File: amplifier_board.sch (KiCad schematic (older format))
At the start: 72 parts, among them J1 external input, J10 external saw, J11 jumper storage, J2 AUDIO, J3 VCC, J4 +5V, J5 GND, J6 -5V, J7 audio tune, J8 speaker, J9 speaker, Q1 SQJ860EP, Q2 Q_NMOS_GSD, Q3 SQJ860EP, U1 AD8038, U2 AD8613, U3 LTC4444-5, U4 AD8468, U5 LM555, U6 AD8038, U7 AD8613

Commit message: up
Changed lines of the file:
@@
 L Device:C C17
 U 1 1 5CAB9B8F
-P 2500 5950
-F 0 "C17" V 2375 5875 50  0000 C CNN
-F 1 "100nF" V 2375 6050 50  0000 C CNN
-F 2 "Capacitors_SMD:C_1206_HandSoldering" H 2538 5800 50  0001 C CNN
-F 3 "~" H 2500 5950 50  0001 C CNN
-	1    2500 5950
+P 3175 5950
+F 0 "C17" V 3050 5875 50  0000 C CNN
+F 1 "100nF" V 3050 6050 50  0000 C CNN
+F 2 "Capacitors_SMD:C_1206_HandSoldering" H 3213 5800 50  0001 C CNN
+F 3 "~" H 3175 5950 50  0001 C CNN
+	1    3175 5950
 	-1   0    0    1
 $EndComp
@@
 L Device:C C18
 U 1 1 5CABA0D0
-P 2750 5950
-F 0 "C18" V 2625 5875 50  0000 C CNN
-F 1 "100nF" V 2625 6050 50  0000 C CNN
-F 2 "Capacitors_SMD:C_1206_HandSoldering" H 2788 5800 50  0001 C CNN
-F 3 "~" H 2750 5950 50  0001 C CNN
-	1    2750 5950
+P 3425 5950
+F 0 "C18" V 3300 5875 50  0000 C CNN
+F 1 "100nF" V 3300 6050 50  0000 C CNN
+F 2 "Capacitors_SMD:C_1206_HandSoldering" H 3463 5800 50  0001 C CNN
+F 3 "~" H 3425 5950 50  0001 C CNN
+	1    3425 5950
 	-1   0    0    1
 $EndComp
@@
 L Device:C C19
 U 1 1 5CABA154
-P 3000 5950
-F 0 "C19" V 2875 5875 50  0000 C CNN
-F 1 "100nF" V 2875 6050 50  0000 C CNN
-F 2 "Capacitors_SMD:C_1206_HandSoldering" H 3038 5800 50  0001 C CNN
-F 3 "~" H 3000 5950 50  0001 C CNN
-	1    3000 5950
+P 3675 5950
+F 0 "C19" V 3550 5875 50  0000 C CNN
+F 1 "100nF" V 3550 6050 50  0000 C CNN
+F 2 "Capacitors_SMD:C_1206_HandSoldering" H 3713 5800 50  0001 C CNN
+F 3 "~" H 3675 5950 50  0001 C CNN
+	1    3675 5950
 	-1   0    0    1
 $EndComp
@@
 L Device:C C16
 U 1 1 5CABD33C
-P 2250 5950
-F 0 "C16" V 2125 5875 50  0000 C CNN
-F 1 "100nF" V 2125 6050 50  0000 C CNN
-F 2 "Capacitors_SMD:C_1206_HandSoldering" H 2288 5800 50  0001 C CNN
-F 3 "~" H 2250 5950 50  0001 C CNN
-	1    2250 5950
+P 2925 5950
+F 0 "C16" V 2800 5875 50  0000 C CNN
+F 1 "100nF" V 2800 6050 50  0000 C CNN
+F 2 "Capacitors_SMD:C_1206_HandSoldering" H 2963 5800 50  0001 C CNN
+F 3 "~" H 2925 5950 50  0001 C CNN
+	1    2925 5950
 	-1   0    0    1
 $EndComp
@@
 $EndComp
 Wire Wire Line
-	3000 5800 2750 5800
+	3675 5800 3425 5800
 Connection ~ 1250 5800
 Wire Wire Line
@@
 Wire Wire Line
 	1750 5800 1500 5800
-Connection ~ 2500 5800
-Wire Wire Line
-	2500 5800 2250 5800
-Connection ~ 2750 5800
-Wire Wire Line
-	2750 5800 2500 5800
+Connection ~ 3175 5800
+Wire Wire Line
+	3175 5800 2925 5800
+Connection ~ 3425 5800
+Wire Wire Line
+	3425 5800 3175 5800
 Wire Wire Line
 	1000 5750 1000 5800
@@
 	1500 6100 1750 6100
 Wire Wire Line
-	2250 6100 2500 6100
-Connection ~ 2500 6100
-Wire Wire Line
-	2500 6100 2750 6100
-Connection ~ 2750 6100
-Wire Wire Line
-	2750 6100 3000 6100
+	2925 6100 3175 6100
+Connection ~ 3175 6100
+Wire Wire Line
+	3175 6100 3425 6100
+Connection ~ 3425 6100
+Wire Wire Line
+	3425 6100 3675 6100
 $Comp
 L Device:C C21
@@
 L Device:C C22
 U 1 1 5CAD2A32
-P 1500 6700
-F 0 "C22" V 1375 6625 50  0000 C CNN
-F 1 "100nF" V 1375 6800 50  0000 C CNN
-F 2 "Capacitors_SMD:C_1206_HandSoldering" H 1538 6550 50  0001 C CNN
-F 3 "~" H 1500 6700 50  0001 C CNN
-	1    1500 6700
+P 2000 5950
+F 0 "C22" V 1875 5875 50  0000 C CNN
+F 1 "100nF" V 1875 6050 50  0000 C CNN
+F 2 "Capacitors_SMD:C_1206_HandSoldering" H 2038 5800 50  0001 C CNN
+F 3 "~" H 2000 5950 50  0001 C CNN
+	1    2000 5950
 	-1   0    0    1
 $EndComp
@@
 L Device:C C23
 U 1 1 5CAD2A39
-P 1750 6700
-F 0 "C23" V 1625 6625 50  0000 C CNN
-F 1 "100nF" V 1625 6800 50  0000 C CNN
-F 2 "Capacitors_SMD:C_1206_HandSoldering" H 1788 6550 50  0001 C CNN
-F 3 "~" H 1750 6700 50  0001 C CNN
-	1    1750 6700
+P 2250 5950
+F 0 "C23" V 2125 5875 50  0000 C CNN
+F 1 "100nF" V 2125 6050 50  0000 C CNN
+F 2 "Capacitors_SMD:C_1206_HandSoldering" H 2288 5800 50  0001 C CNN
+F 3 "~" H 2250 5950 50  0001 C CNN
+	1    2250 5950
 	-1   0    0    1
 $EndComp
@@
 $EndComp
 Wire Wire Line
-	1750 6550 1500 6550
-Connection ~ 1250 6550
+	2250 5800 2000 5800
 Wire Wire Line
 	1250 6550 1000 6550
-Connection ~ 1500 6550
-Wire Wire Line
-	1500 6550 1250 6550
+Connection ~ 2000 5800
+Wire Wire Line
+	2000 5800 1750 5800
 Wire Wire Line
 	1000 6850 1250 6850
-Connection ~ 1250 6850
-Wire Wire Line
-	1250 6850 1500 6850
-Connection ~ 1500 6850
-Wire Wire Line
-	1500 6850 1750 6850
+Wire Wire Line
+	1750 6100 2000 6100
+Connection ~ 2000 6100
+Wire Wire Line
+	2000 6100 2250 6100
 $Comp
 L power:GND #PWR0135
@@
 L power:+5V #PWR0101
 U 1 1 5CCBC421
-P 2250 5750
-F 0 "#PWR0101" H 2250 5600 50  0001 C CNN
-F 1 "+5V" H 2200 5900 50  0000 C CNN
-F 2 "" H 2250 5750 50  0001 C CNN
-F 3 "" H 2250 5750 50  0001 C CNN
-	1    2250 5750
+P 2925 5750
+F 0 "#PWR0101" H 2925 5600 50  0001 C CNN
+F 1 "+5V" H 2875 5900 50  0000 C CNN
+F 2 "" H 2925 5750 50  0001 C CNN
+F 3 "" H 2925 5750 50  0001 C CNN
+	1    2925 5750
 	1    0    0    -1
 $EndComp
@@
 L power:-5V #PWR0145
 U 1 1 5CCBC4BA
-P 2250 6150
-F 0 "#PWR0145" H 2250 6250 50  0001 C CNN
-F 1 "-5V" H 2300 6275 50  0000 C CNN
-F 2 "" H 2250 6150 50  0001 C CNN
-F 3 "" H 2250 6150 50  0001 C CNN
-	1    2250 6150
-	-1   0    0    1
-$EndComp
-Wire Wire Line
-	2250 5750 2250 5800
-Connection ~ 2250 5800
-Connection ~ 2250 6100
-Wire Wire Line
-	2250 6100 2250 6150
+P 2925 6150
+F 0 "#PWR0145" H 2925 6250 50  0001 C CNN
+F 1 "-5V" H 2975 6275 50  0000 C CNN
+F 2 "" H 2925 6150 50  0001 C CNN
+F 3 "" H 2925 6150 50  0001 C CNN
+	1    2925 6150
+	-1   0    0    1
+$EndComp
+Wire Wire Line
+	2925 5750 2925 5800
+Connection ~ 2925 5800
+Connection ~ 2925 6100
+Wire Wire Line
+	2925 6100 2925 6150
 Wire Wire Line
 	1700 1450 2450 1450
@@
 	10325 3675 10325 3825
 $Comp
-L power:GND #PWR?
+L power:GND #PWR0146
 U 1 1 5CCF3D0D
 P 9925 3825
-F 0 "#PWR?" H 9925 3575 50  0001 C CNN
+F 0 "#PWR0146" H 9925 3575 50  0001 C CNN
 F 1 "GND" H 9930 3652 50  0000 C CNN
 F 2 "" H 9925 3825 50  0001 C CNN
@@
 Wire Wire Line
 	9925 3825 9925 3775
+Connection ~ 1750 5800
+Connection ~ 1750 6100
 $EndSCHEMATC

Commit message: more files
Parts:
- added C24, C25: 100nF, Capacitor_SMD:C_1206_3216Metric_Pad1.42x1.75mm_HandSolder, symbol amplifier_board-rescue:C-Device
- added JP4: internal audio, Connector_PinHeader_2.54mm:PinHeader_1x02_P2.54mm_Vertical, symbol amplifier_board-rescue:Jumper-Device
- C1: symbol Device:CP -> amplifier_board-rescue:CP-Device
- C10, C11, C12, C13, C14, C15, C16, C17, C18, C19, C2, C20, C21, C22, C23, C3, C4, C5, C6, C7, C8, C9: symbol Device:C -> amplifier_board-rescue:C-Device
- D1, D2, D3: symbol Device:D_Schottky -> amplifier_board-rescue:D_Schottky-Device
- J1, J10, J7, J9: symbol Connector:Conn_Coaxial -> amplifier_board-rescue:Conn_Coaxial-Connector
- J11: symbol Connector_Generic:Conn_02x03_Counter_Clockwise -> amplifier_board-rescue:Conn_02x03_Counter_Clockwise-Connector_Generic
- J2: symbol Connector_Generic:Conn_01x03 -> amplifier_board-rescue:Conn_01x03-Connector_Generic
- J3, J4, J5, J6: symbol Connector:Conn_01x01_Female -> amplifier_board-rescue:Conn_01x01_Female-Connector
- J8: symbol Connector:Screw_Terminal_01x02 -> amplifier_board-rescue:Screw_Terminal_01x02-Connector
- JP1, JP2: symbol Device:Jumper -> amplifier_board-rescue:Jumper-Device
- JP3: symbol Device:Jumper_NO_Small -> amplifier_board-rescue:Jumper_NO_Small-Device
- L1: symbol Device:L -> amplifier_board-rescue:L-Device
- Q1, Q3: symbol Transistor_FET:Si7336ADP -> amplifier_board-rescue:Si7336ADP-Transistor_FET
- Q2: symbol Device:Q_NMOS_GSD -> amplifier_board-rescue:Q_NMOS_GSD-Device
- R1, R10, R11, R12, R13, R14, R15, R16, R17, R2, R3, R4, R5, R6, R7, R8, R9: symbol Device:R -> amplifier_board-rescue:R-Device
- RV1, RV4: symbol Device:R_POT -> amplifier_board-rescue:R_POT-Device
- RV2, RV3: symbol Device:R_POT_Dual -> amplifier_board-rescue:R_POT_Dual-Device
- U1, U6: symbol Amplifier_Operational:AD8001AR -> amplifier_board-rescue:AD8001AR-Amplifier_Operational
- U2, U7: symbol Amplifier_Operational:MCP6561-OT -> amplifier_board-rescue:MCP6561-OT-Amplifier_Operational
- U5: symbol Timer:LM555 -> amplifier_board-rescue:LM555-Timer
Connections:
- wire segments 188 -> 193

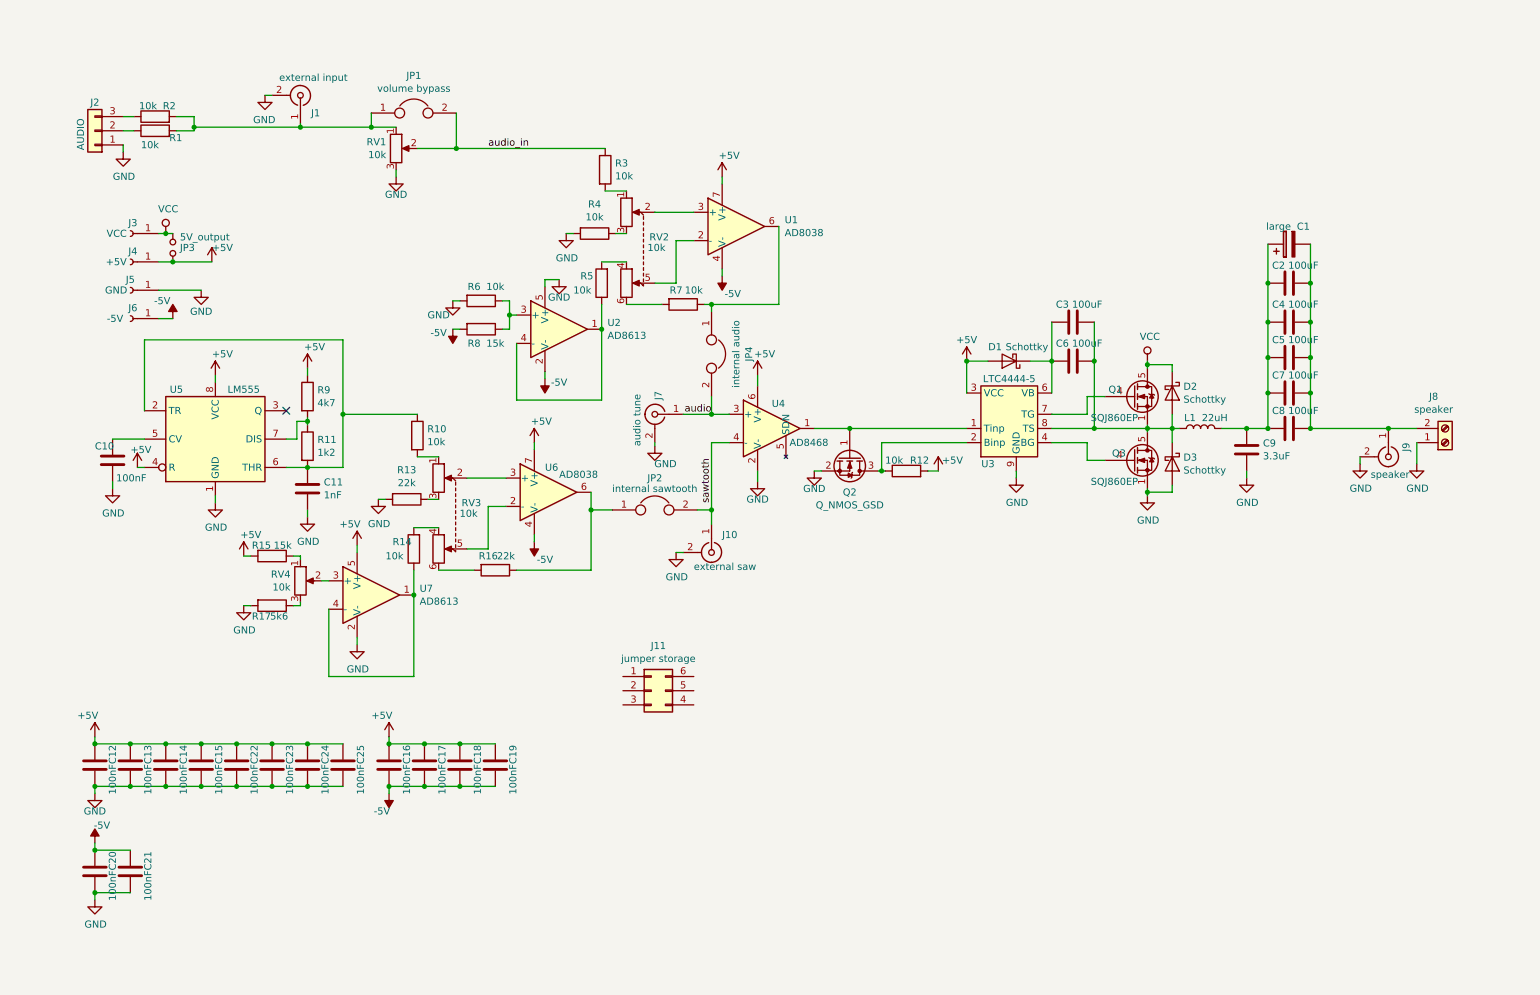
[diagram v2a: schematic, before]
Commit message: aaa
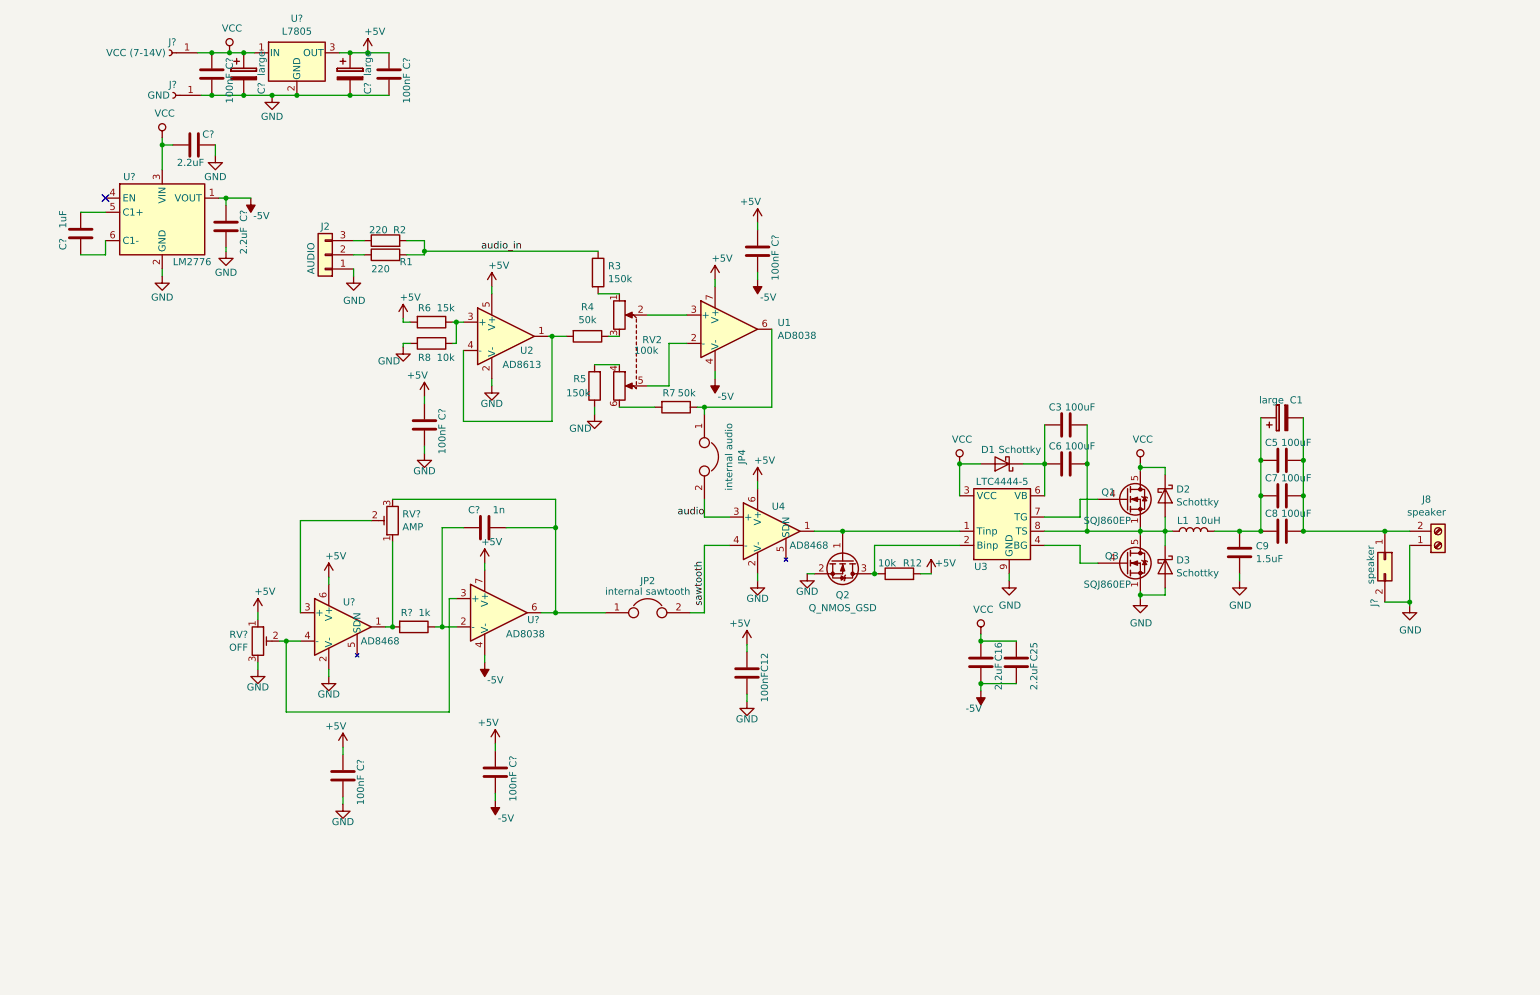
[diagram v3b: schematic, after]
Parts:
- removed C10, C13, C14, C15, C17, C18, C19, C20, C21, C22, C23: 100nF, Capacitors_SMD:C_1206_HandSoldering, symbol amplifier_board-rescue:C-Device
- removed C11: 1nF, Capacitors_SMD:C_1206_HandSoldering, symbol amplifier_board-rescue:C-Device
- removed C2, C4: 100uF, Capacitors_SMD:C_1206_HandSoldering, symbol amplifier_board-rescue:C-Device
- removed C24: 100nF, Capacitor_SMD:C_1206_3216Metric_Pad1.42x1.75mm_HandSolder, symbol amplifier_board-rescue:C-Device
- removed J1: external input, Connect:BNC, symbol amplifier_board-rescue:Conn_Coaxial-Connector
- removed J10: external saw, Connect:BNC, symbol amplifier_board-rescue:Conn_Coaxial-Connector
- removed J11: jumper storage, Pin_Headers:Pin_Header_Straight_2x03_Pitch2.54mm, symbol amplifier_board-rescue:Conn_02x03_Counter_Clockwise-Connector_Generic
- removed J3: VCC, Mounting_Holes:MountingHole_4mm_Pad, symbol amplifier_board-rescue:Conn_01x01_Female-Connector
- removed J4: +5V, Mounting_Holes:MountingHole_4mm_Pad, symbol amplifier_board-rescue:Conn_01x01_Female-Connector
- removed J5: GND, Mounting_Holes:MountingHole_4mm_Pad, symbol amplifier_board-rescue:Conn_01x01_Female-Connector
- removed J6: -5V, Mounting_Holes:MountingHole_4mm_Pad, symbol amplifier_board-rescue:Conn_01x01_Female-Connector
- removed J7: audio tune, Connect:BNC, symbol amplifier_board-rescue:Conn_Coaxial-Connector
- removed J9: speaker, Connect:BNC, symbol amplifier_board-rescue:Conn_Coaxial-Connector
- removed JP1: volume bypass, Pin_Headers:Pin_Header_Straight_1x02_Pitch2.54mm, symbol amplifier_board-rescue:Jumper-Device
- removed JP3: 5V_output, Pin_Headers:Pin_Header_Straight_1x02_Pitch2.54mm, symbol amplifier_board-rescue:Jumper_NO_Small-Device
- removed R10, R14: 10k, Resistors_SMD:R_1206_HandSoldering, symbol amplifier_board-rescue:R-Device
- removed R11: 1k2, Resistors_SMD:R_1206_HandSoldering, symbol amplifier_board-rescue:R-Device
- removed R13, R16: 22k, Resistors_SMD:R_1206_HandSoldering, symbol amplifier_board-rescue:R-Device
- removed R15: 15k, Resistors_SMD:R_1206_HandSoldering, symbol amplifier_board-rescue:R-Device
- removed R17: 5k6, Resistors_SMD:R_1206_HandSoldering, symbol amplifier_board-rescue:R-Device
- removed R9: 4k7, Resistors_SMD:R_1206_HandSoldering, symbol amplifier_board-rescue:R-Device
- removed RV1, RV4: 10k, Potentiometers:Potentiometer_Alps_RK163_Single_Vertical, symbol amplifier_board-rescue:R_POT-Device
- removed RV3: 10k, Potentiometers:Potentiometer_Alps_RK163_Double_Vertical, symbol amplifier_board-rescue:R_POT_Dual-Device
- removed U5: LM555, Housings_SOIC:SOIC-8_3.9x4.9mm_Pitch1.27mm, symbol amplifier_board-rescue:LM555-Timer
- removed U6: AD8038, Housings_SOIC:SOIC-8_3.9x4.9mm_Pitch1.27mm, symbol amplifier_board-rescue:AD8001AR-Amplifier_Operational
- removed U7: AD8613, TO_SOT_Packages_SMD:SOT-23-5_HandSoldering, symbol amplifier_board-rescue:MCP6561-OT-Amplifier_Operational
- added C?: 1n, Capacitors_SMD:C_1206_HandSoldering, symbol amplifier_board-rescue:C-Device
- added C? (x2): large, Capacitors_ThroughHole:CP_Radial_D10.0mm_P2.50mm_P5.00mm, symbol amplifier_board-rescue:CP-Device
- added C? (x6): 100nF, Capacitors_SMD:C_1206_HandSoldering, symbol amplifier_board-rescue:C-Device
- added C? (x2): 2.2uF, Capacitors_SMD:C_1206_HandSoldering, symbol amplifier_board-rescue:C-Device
- added C?: 1uF, Capacitors_SMD:C_1206_HandSoldering, symbol amplifier_board-rescue:C-Device
- added J?: speaker, symbol Connector_Generic:Conn_02x01
- added J?: VCC (7-14V), Mounting_Holes:MountingHole_4mm_Pad, symbol amplifier_board-rescue:Conn_01x01_Female-Connector
- added J?: GND, Mounting_Holes:MountingHole_4mm_Pad, symbol amplifier_board-rescue:Conn_01x01_Female-Connector
- added R?: 1k, Resistors_SMD:R_1206_HandSoldering, symbol amplifier_board-rescue:R-Device
- added RV?: OFF, symbol Device:R_POT_TRIM
- added RV?: AMP, symbol Device:R_POT_TRIM
- added U?: AD8468, TO_SOT_Packages_SMD:SOT-363_SC-70-6_Handsoldering, symbol AD8468:AD8468
- added U?: AD8038, Housings_SOIC:SOIC-8_3.9x4.9mm_Pitch1.27mm, symbol amplifier_board-rescue:AD8001AR-Amplifier_Operational
- added U?: L7805, symbol Regulator_Linear:L7805
- added U?: LM2776, Package_TO_SOT_SMD:SOT-23-6, symbol Regulator_SwitchedCapacitor:LM2776
- C16, C25: value 100nF -> 2.2uF
- C9: value 3.3uF -> 1.5uF
- L1: value 22uH -> 10uH
- R1, R2: value 10k -> 220
- R3, R5: value 10k -> 150k
- R4, R7: value 10k -> 50k
- R6: value 10k -> 15k
- R8: value 15k -> 10k
- RV2: value 10k -> 100k
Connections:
- net +5V: now also R6.2, U2.5 (V+), C?.1, C?.2, C?.2, C?.2, C?.2, C?.2, RV?.1, U?.3 (OUT), U?.6 (V+), U?.7 (V+); no longer C16.2, C25.2, D1.2 (A), U3.3 (VCC)
- net -5V: now also C25.1, C?.1, C?.1, C?.2, U?.1 (VOUT), U?.4 (V-); no longer R8.2, U2.2 (V-)
- net GND: now also R5.1, R8.2, U2.2 (V-), C?.1, C?.1, C?.1, C?.1, C?.1, C?.2, C?.2, C?.2, J?.1 (Pin_1), J?.2 (Pin_2), RV?.3, U?.2 (GND), U?.2 (GND), U?.2 (V-); no longer C25.1, R4.2, R6.2, U2.5 (V+)
- net VCC: now also C16.2, C25.2, D1.2 (A), U3.3 (VCC), C?.1, C?.1, C?.2, J?.1 (Pin_1), U?.1 (IN), U?.3 (VIN)
- net audio_in: now also R1.2, R2.2
- net at JP2.1: now also C?.1, RV?.3, U?.6
- net at U2.1, U2.4 (-): now also R4.2; no longer R5.1
- net at C1.2, C5.1, C7.1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: now also J?.1 (Pin_1)
- new net: R?.2, RV?.1, U?.1
- new net: RV?.2, U?.3 (+)
- new net: RV?.2, U?.3 (+), U?.4 (-)
- new net: C?.2, R?.1, U?.2 (-)
- new net: C?.1, U?.5 (C1+)
- new net: C?.2, U?.6 (C1-)
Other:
- moved on the sheet: C1, C12, C16, C25, C3, C5, C6, C7, C8, C9, D1, D2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
